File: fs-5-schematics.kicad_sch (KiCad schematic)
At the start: 13 parts, among them J1 12V, J2 5V, U1 TPS54202DDC

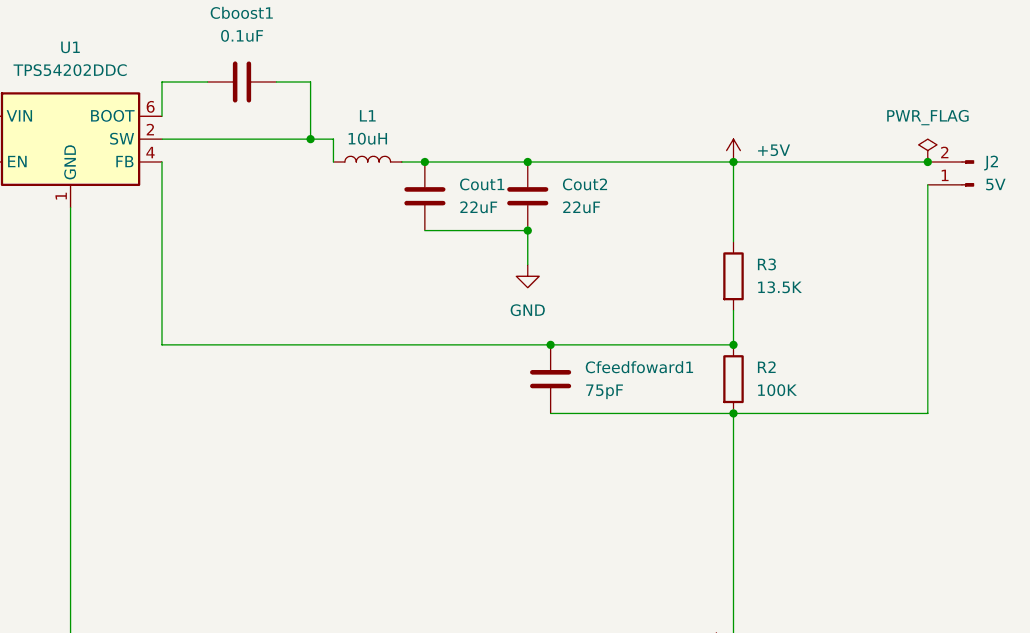
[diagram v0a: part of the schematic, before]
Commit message: PCb layouts complete?, need checked
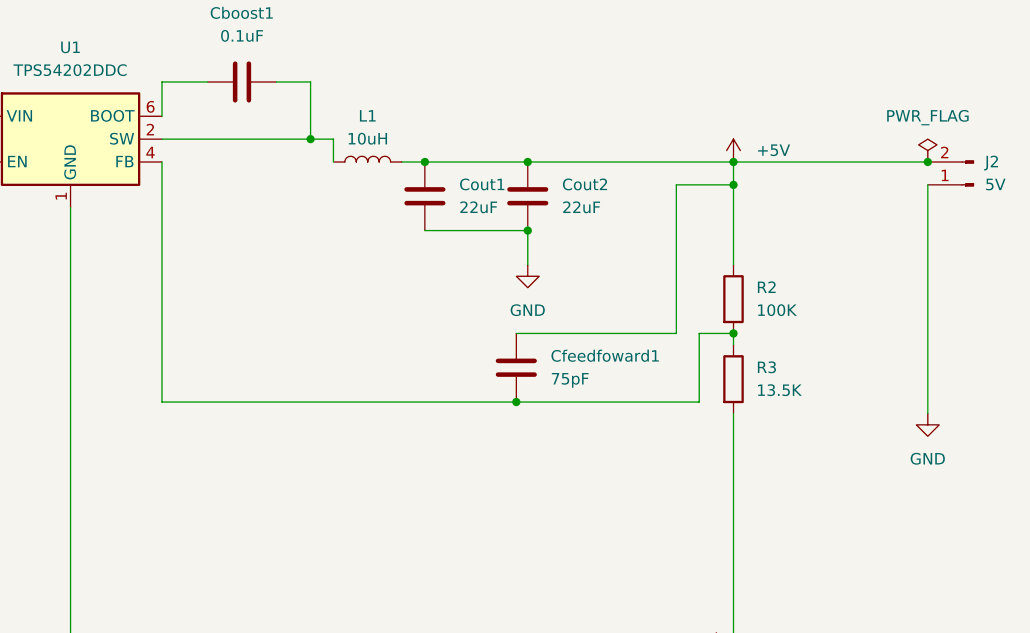
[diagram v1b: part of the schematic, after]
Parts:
- J1, J2: footprint (none) -> TerminalBlock:TerminalBlock_MaiXu_MX126-5.0-02P_1x02_P5.00mm
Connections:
- net +5V: now also Cfeedfoward1.1, R2.1; no longer R3.1
- net GND: now also R3.2; no longer Cfeedfoward1.2, R2.2
- new net: Cfeedfoward1.2, R2.2, R3.1, U1.4 (FB)
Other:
- moved on the sheet: Cfeedfoward1, R2
